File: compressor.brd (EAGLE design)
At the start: 160 x 100 mm, 46 parts, among them U1 MAX5419LETA+, U2 MAX5419LETA+, U3 LM4562MAX/NOPB, U4 LM4562MAX/NOPB, U5 LM4562MAX/NOPB, U6 LM4562MAX/NOPB

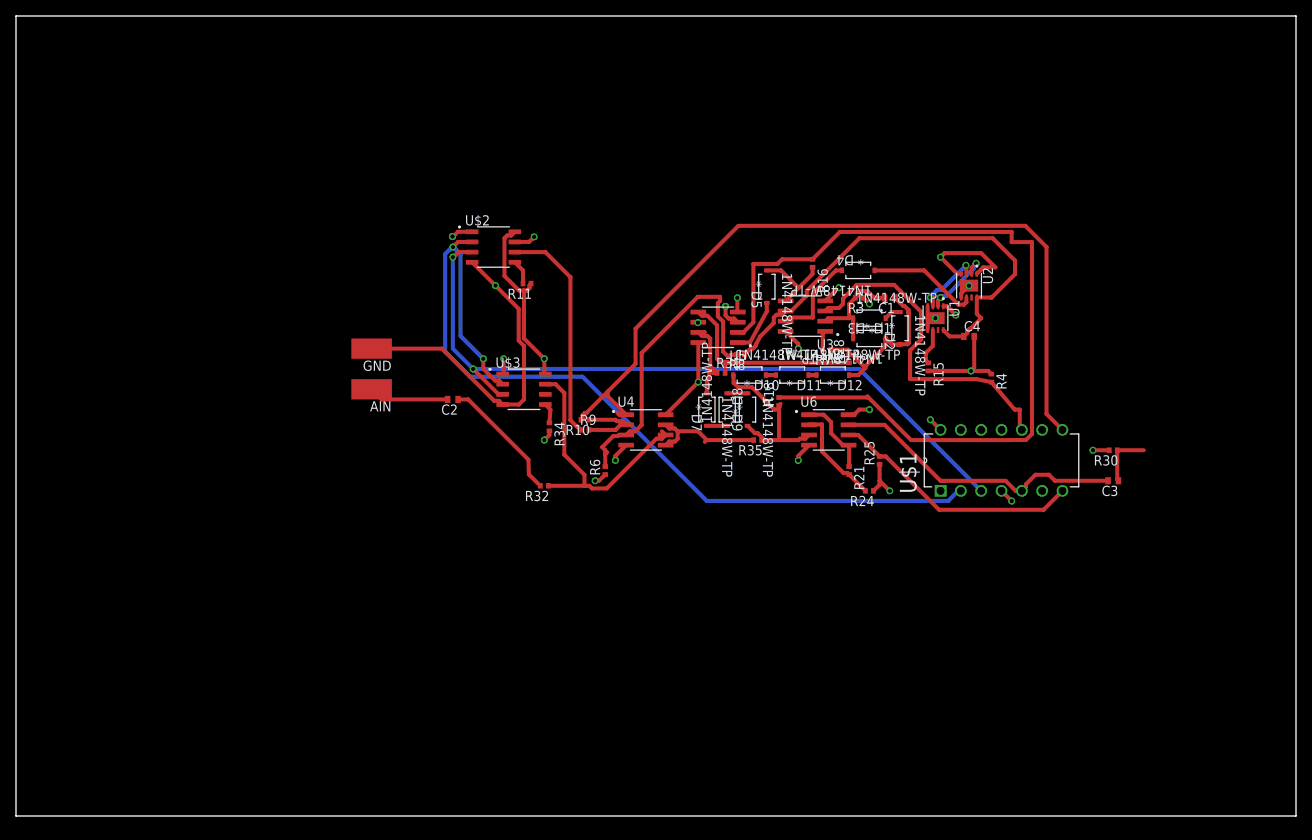
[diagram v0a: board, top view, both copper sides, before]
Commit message: corrections
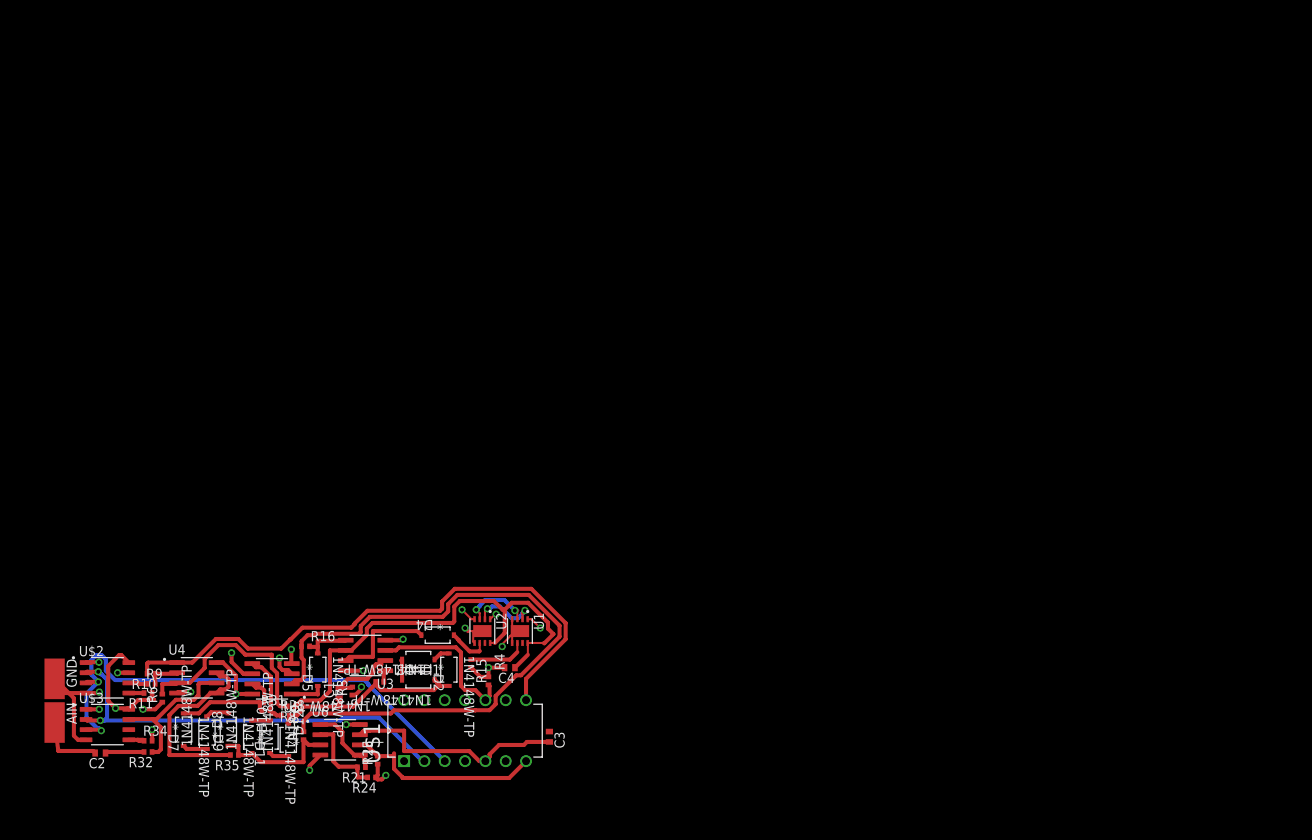
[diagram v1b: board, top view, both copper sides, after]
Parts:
- removed R30: 1M, rcl:R0402
- C2: value 0.1 -> 0.1u
- moved C1 84.7 mm to (40.4, 15.4), turned to 90 degrees
- moved R28 83.4 mm to (33.7, 12.6), turned to 0 degrees
- moved D12 81.9 mm to (34.0, 9.53), turned to 90 degrees
- moved R3 80.2 mm to (42.0, 15.6), turned to 90 degrees
- moved R16 79.4 mm to (36.2, 21.2), turned to 0 degrees
- moved D11 79.4 mm to (31.8, 9.91), turned to 270 degrees
- moved C3 77.4 mm to (66.7, 9.91), turned to 270 degrees
- moved D10 76.9 mm to (29.5, 9.91), turned to 90 degrees
- moved D7 76.7 mm to (21.0, 10.8)
- moved D8 76.5 mm to (23.9, 10.4)
- moved R35 76.3 mm to (27.3, 7.62)
- moved D9 76.2 mm to (26.5, 10.8)
- moved U$1 75.1 mm to (63.8, 14.5)
- moved U2 74.6 mm to (58.3, 23.1)
- moved D5 73.8 mm to (37.7, 18.3)
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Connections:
- net AOUT: no longer R30.1
- net VSS: no longer R30.2
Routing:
- net VSS: track 225.5 -> 130.6 mm, vias 9 -> 7
- net SCK: track 109.0 -> 53.6 mm
- net PA0: track 100.8 -> 72.5 mm
- net SDI/O: track 92.5 -> 65.0 mm
- net P0W_0: track 27.9 -> 2.34 mm
- net VREF: track 172.1 -> 147.2 mm
- net PB0: track 42.1 -> 20.1 mm
- net N$16: track 105.8 -> 84.2 mm
- net N$8: track 25.4 -> 9.03 mm
- net VDD: track 133.6 -> 118.8 mm
- net P0B_1: track 33.7 -> 19.2 mm
- net N$6: track 39.9 -> 25.9 mm
- net N$30: track 15.8 -> 4.87 mm
- net N$27: track 14.9 -> 24.6 mm
- net PB1: track 37.2 -> 28.2 mm
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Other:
- board outline removed

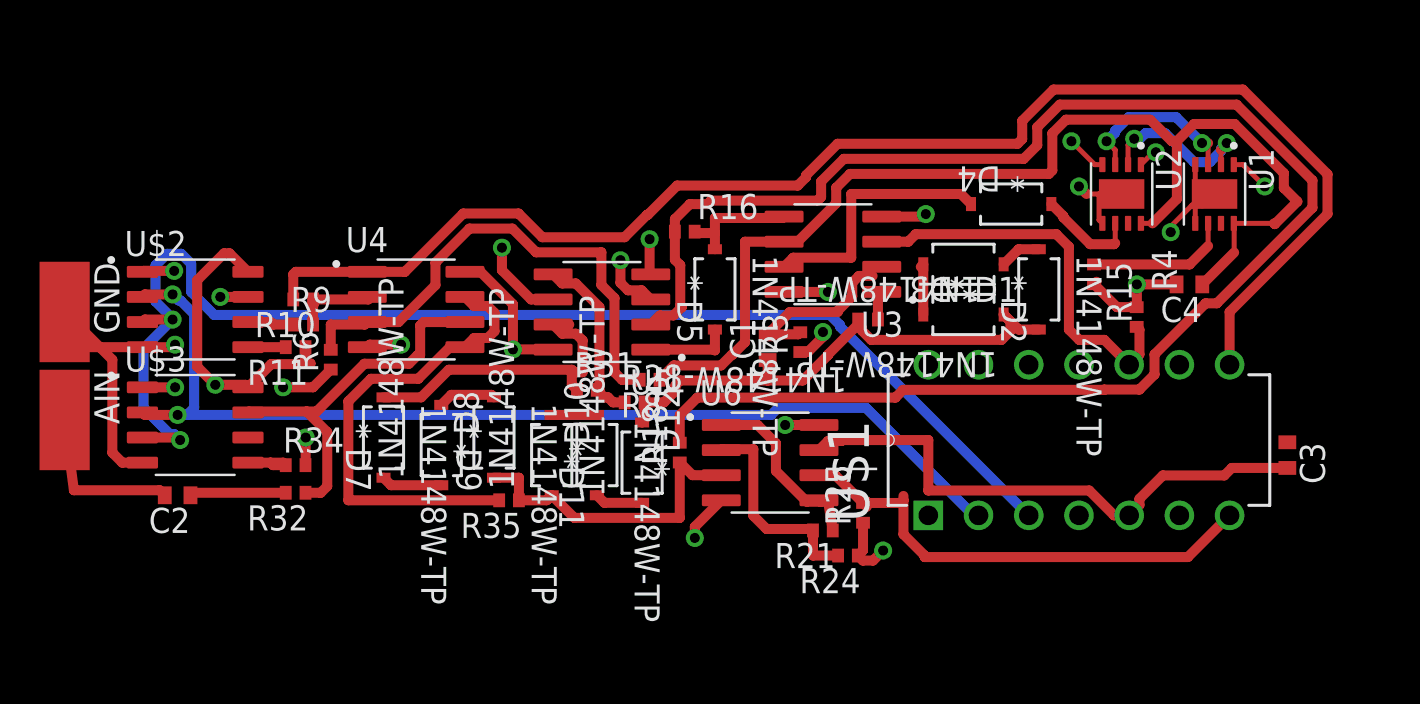
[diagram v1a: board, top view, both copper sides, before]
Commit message: updates
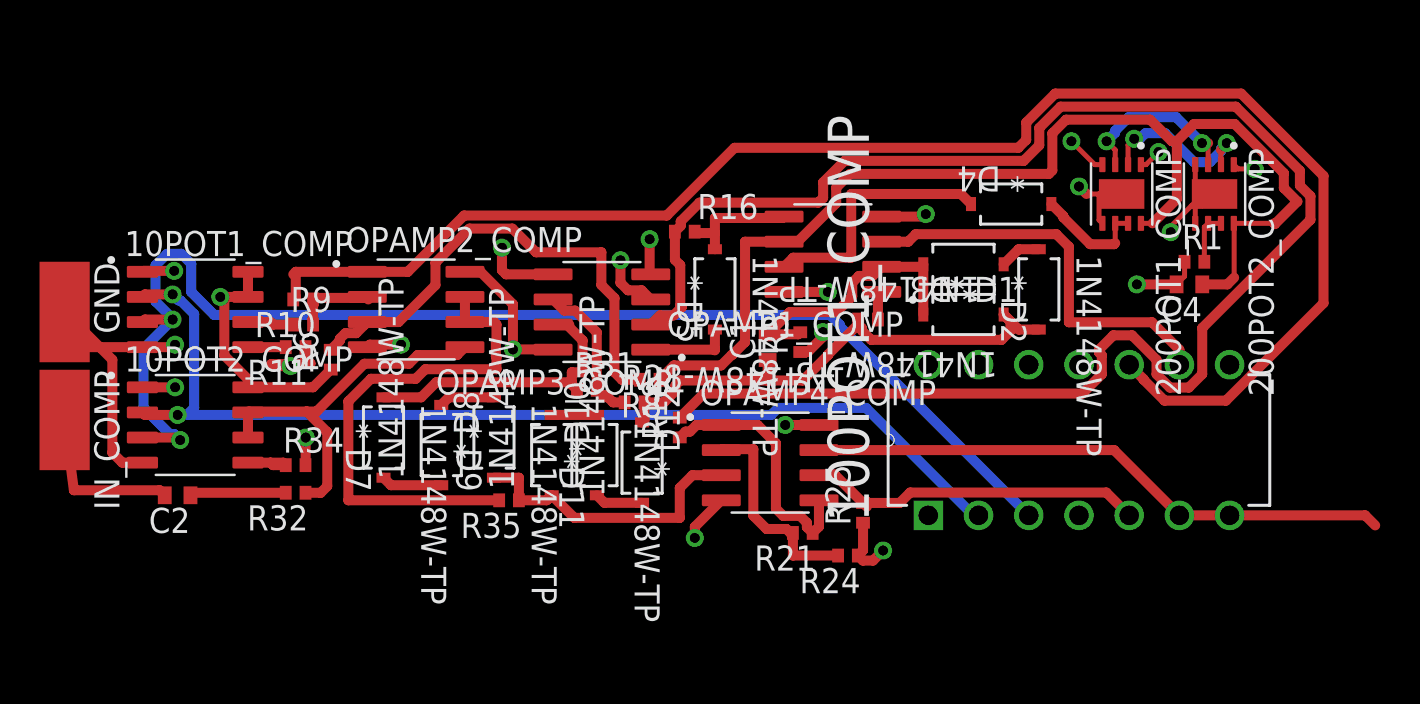
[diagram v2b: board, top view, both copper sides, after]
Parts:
- removed C3: 1.5u, rcl:C0402
- removed R15: 100k, rcl:R0402
- removed R4: 10k, rcl:R0402
- added R1: 100k, rcl:R0402
- C2: value 0.1u -> 10u
- moved R18 1.27 mm to (35.9, 11.3)
- moved R21 1.02 mm to (42.2, 5.97)
- renumbered AIN to IN_COMP, U$1 to 100POT1_COMP, U$2 to 10POT1_COMP, U$3 to 10POT2_COMP, U1 to 200POT2_COMP, U2 to 200POT1_COMP, U3 to OPAMP1_COMP, U4 to OPAMP2_COMP, U5 to OPAMP3_COMP, U6 to OPAMP4_COMP
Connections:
- net AIN renamed IN_COMP
- net CS0 renamed CS0_COMP
- net CS1 renamed CS1_COMP
- net CS2 renamed CS2_COMP
- net H_0 renamed H1_COMP
- net N$1 renamed OUT_A1_COMP
- net N$14 renamed OUT_B1_COMP
- net N$15 renamed POS_B1_COMP
- net N$16 renamed NEG_A3_COMP
- net N$19 renamed NEG_A4_COMP
- net N$2 renamed OUT_B3_COMP
- net N$3 renamed NEG_A1_COMP
- net N$4 renamed OUT_A3_COMP
- net N$6 renamed POS_A2_COMP
- net N$7 renamed NEG_A2_COMP
- net P0A_0 renamed P0A1_COMP
- net P0A_1 renamed P0A2_COMP
- net P0W_0 renamed P0W1_COMP
- net SCL renamed SCL_COMP
- net SDA renamed SDA_COMP
- net VSS renamed GND
- removed net AOUT: C3.1
- removed net L_0: 200POT2_COMP.6, R15.1
- removed net L_1: 200POT1_COMP.6, D4.C
- removed net N$18: OPAMP4_COMP.1, OPAMP4_COMP.5, R21.1
- removed net N$26: D10.C, D9.A, OPAMP4_COMP.3, R18.1, R35.1
- removed net N$27: OPAMP2_COMP.5, OPAMP2_COMP.7, R35.2
- removed net N$8: OPAMP3_COMP.5, R28.1, R31.2
- removed net P0B_1: 10POT2_COMP.7, OPAMP2_COMP.6, R32.1
- removed net PA0: 100POT1_COMP.8, OPAMP2_COMP.1, R10.2
- removed net PA1: 100POT1_COMP.7, OPAMP4_COMP.6, R25.2
- removed net PB0: 100POT1_COMP.10, OPAMP1_COMP.3, R4.2
- removed net PB1: 100POT1_COMP.5, C3.2, OPAMP4_COMP.7
- removed net RS: 100POT1_COMP.11
- removed net SHDN: 100POT1_COMP.12
- new net L1_COMP: 200POT1_COMP.6, 200POT1_COMP.7, D4.C
- new net L2_COMP: 200POT2_COMP.6, 200POT2_COMP.7, R1.2
- new net NEG_B2_COMP: OPAMP2_COMP.6, OPAMP2_COMP.7, R35.2
- new net NEG_B3_COMP: OPAMP3_COMP.6, R28.1, R31.2
- new net NEG_B4_COMP: 100POT1_COMP.5, OPAMP4_COMP.6, R25.2
- new net OUT_A2_COMP: 100POT1_COMP.10, OPAMP2_COMP.1, R10.2
- new net OUT_A4_COMP: OPAMP4_COMP.1, OPAMP4_COMP.5, R18.1, R21.1
- new net OUT_COMP: 100POT1_COMP.6, 100POT1_COMP.7, OPAMP4_COMP.7
- new net POS_A1_COMP: 100POT1_COMP.9, OPAMP1_COMP.3
- new net POS_A4_COMP: D10.C, D9.A, OPAMP4_COMP.3, R35.1
- new net POS_B2_COMP: 10POT2_COMP.6, 10POT2_COMP.7, OPAMP2_COMP.5, R32.1
- net VDD: no longer 100POT1_COMP.14, 10POT1_COMP.8, 10POT2_COMP.8, 200POT1_COMP.1, 200POT1_COMP.4, 200POT2_COMP.1
- net VREF: now also 100POT1_COMP.11, 100POT1_COMP.12, 100POT1_COMP.14, 100POT1_COMP.8, 10POT1_COMP.8, 10POT2_COMP.8, 200POT1_COMP.1, 200POT1_COMP.4, 200POT2_COMP.1, OPAMP3_COMP.5, R1.1; no longer OPAMP3_COMP.6, R15.2, R4.1
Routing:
- net OUT_A2_COMP: track 0.00 -> 78.7 mm
- net PA0: track 72.5 -> 0.00 mm
- net VDD: track 118.8 -> 51.7 mm, vias 7 -> 4
- net OUT_COMP: track 0.00 -> 29.7 mm
- net PB1: track 28.2 -> 0.00 mm
- net NEG_B2_COMP: track 0.00 -> 26.0 mm
- net PA1: track 25.1 -> 0.00 mm
- net N$27: track 24.6 -> 0.00 mm
- net VREF: track 147.2 -> 170.3 mm, vias 8 -> 10
- net POS_A1_COMP: track 0.00 -> 20.6 mm
- net PB0: track 20.1 -> 0.00 mm
- net POS_B2_COMP: track 0.00 -> 19.4 mm
- net P0B_1: track 19.2 -> 0.00 mm
- net NEG_B4_COMP: track 0.00 -> 17.4 mm
- net N$26: track 16.3 -> 0.00 mm
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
